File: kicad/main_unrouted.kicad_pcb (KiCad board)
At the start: 2 copper layers, 119.4 x 99.1 mm, 41 parts, among them J1 Barrel_Jack, SW1 Reset, SW6 SW_DIP_x08, U1 KM1810VM88, U10 L7805, U11 15 MHz, U12 8255, U13 74HC273, U14 74HC244, U2 W27C512, U3 AS6C4008-55PCN, U4 74HC573, U5 74HC573, U6 ATF16V8, U7 DS1813-5+, U8 74HC00

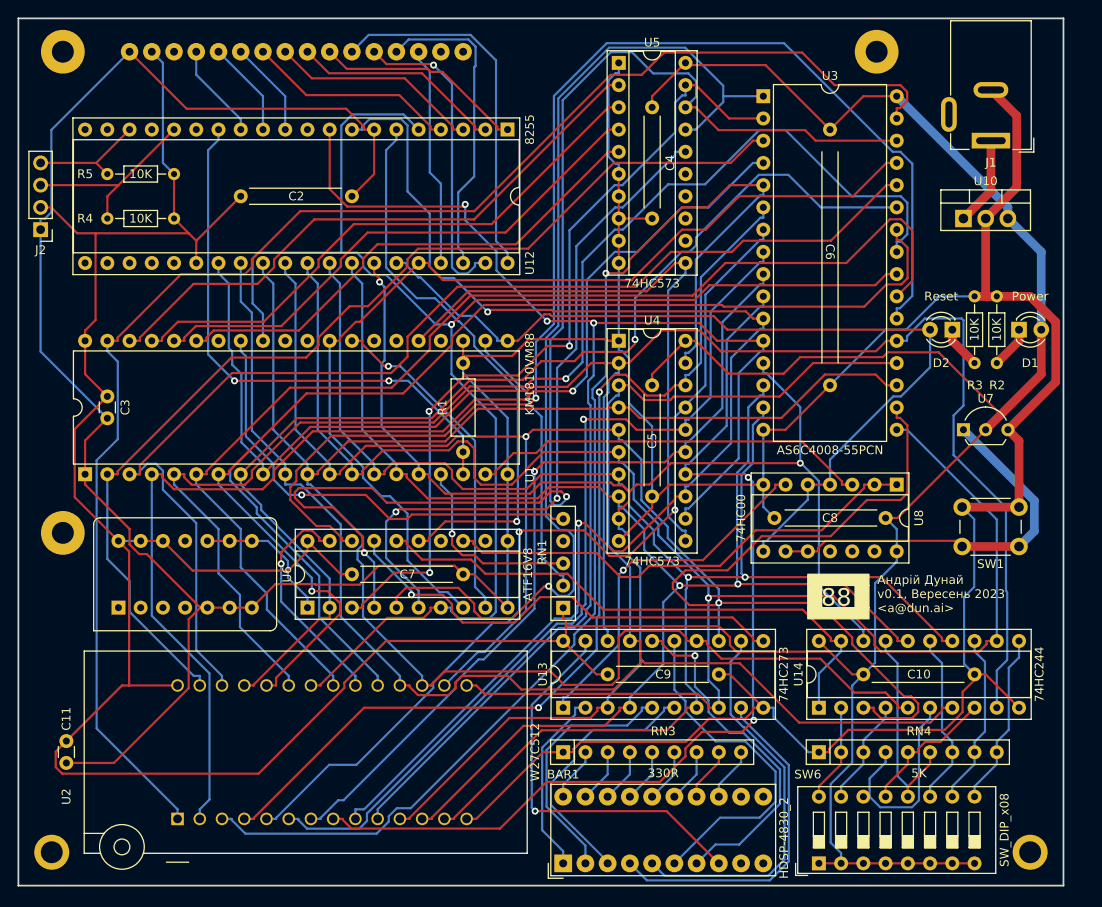
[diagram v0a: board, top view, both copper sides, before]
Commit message: Corrected version of v1 PCB
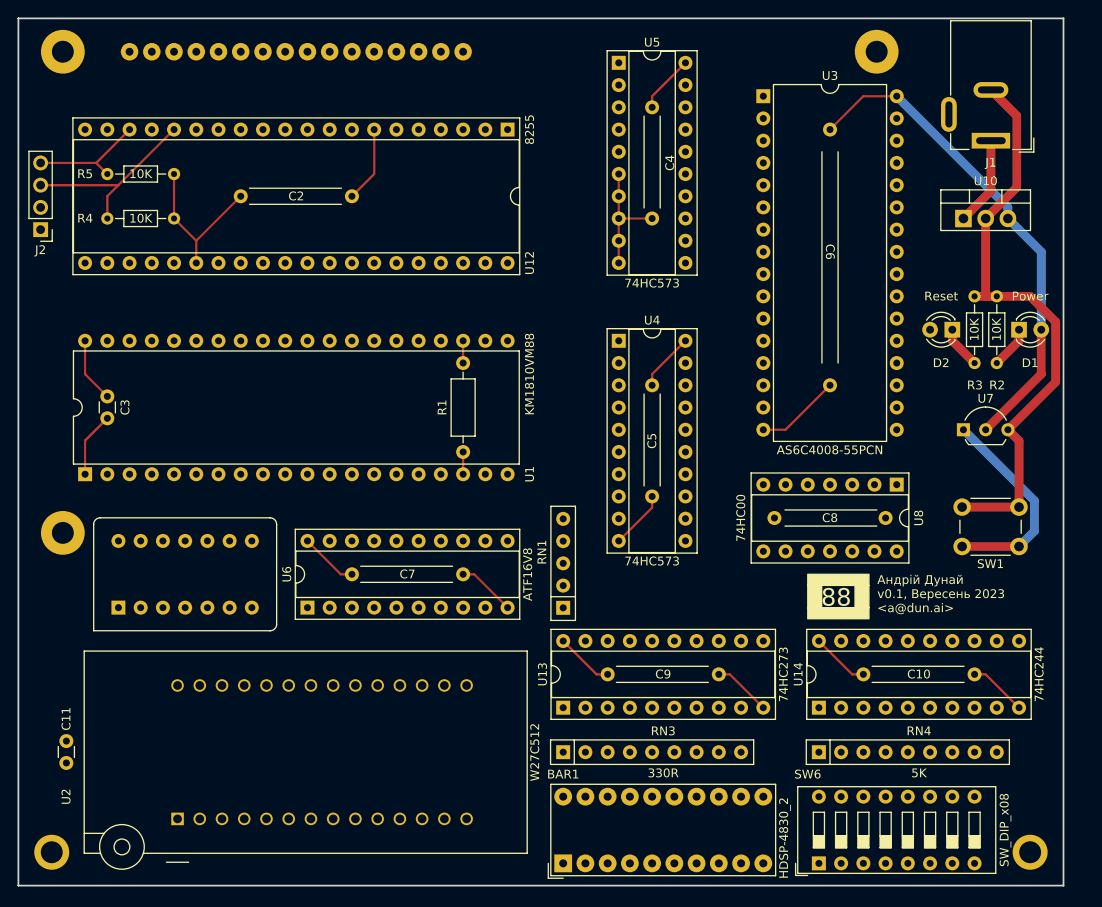
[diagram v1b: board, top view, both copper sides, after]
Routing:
- net GND: track 528.8 -> 137.4 mm
- net +5V: track 482.1 -> 115.9 mm
- net AD_{7}: track 231.3 -> 0.00 mm
- net AD_{4}: track 208.0 -> 0.00 mm, vias 2 -> 0
- net AD_{5}: track 196.6 -> 0.00 mm
- net AD_{6}: track 196.3 -> 0.00 mm
- net AD_{3}: track 194.8 -> 0.00 mm, vias 1 -> 0
- net AD_{2}: track 176.7 -> 0.00 mm, vias 2 -> 0
- net ~{RD}: track 175.7 -> 0.00 mm, vias 1 -> 0
- net A_{15}: track 171.3 -> 0.00 mm
- net AD_{0}: track 167.7 -> 0.00 mm, vias 2 -> 0
- net AD_{1}: track 166.1 -> 0.00 mm, vias 2 -> 0
- net A_{0}: track 158.5 -> 0.00 mm, vias 3 -> 0
- net A_{1}: track 152.0 -> 0.00 mm, vias 2 -> 0
- net A_{17}: track 148.6 -> 0.00 mm, vias 2 -> 0
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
